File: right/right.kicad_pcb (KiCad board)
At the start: 2 copper layers, 50 parts, among them J2 USB_C_Receptacle_OUT, SW1 SW_Push, SW2 SW_SPDT, U1 STM32G0B1CBTx, U2 SRV05-4, U3 XC6206P332MR

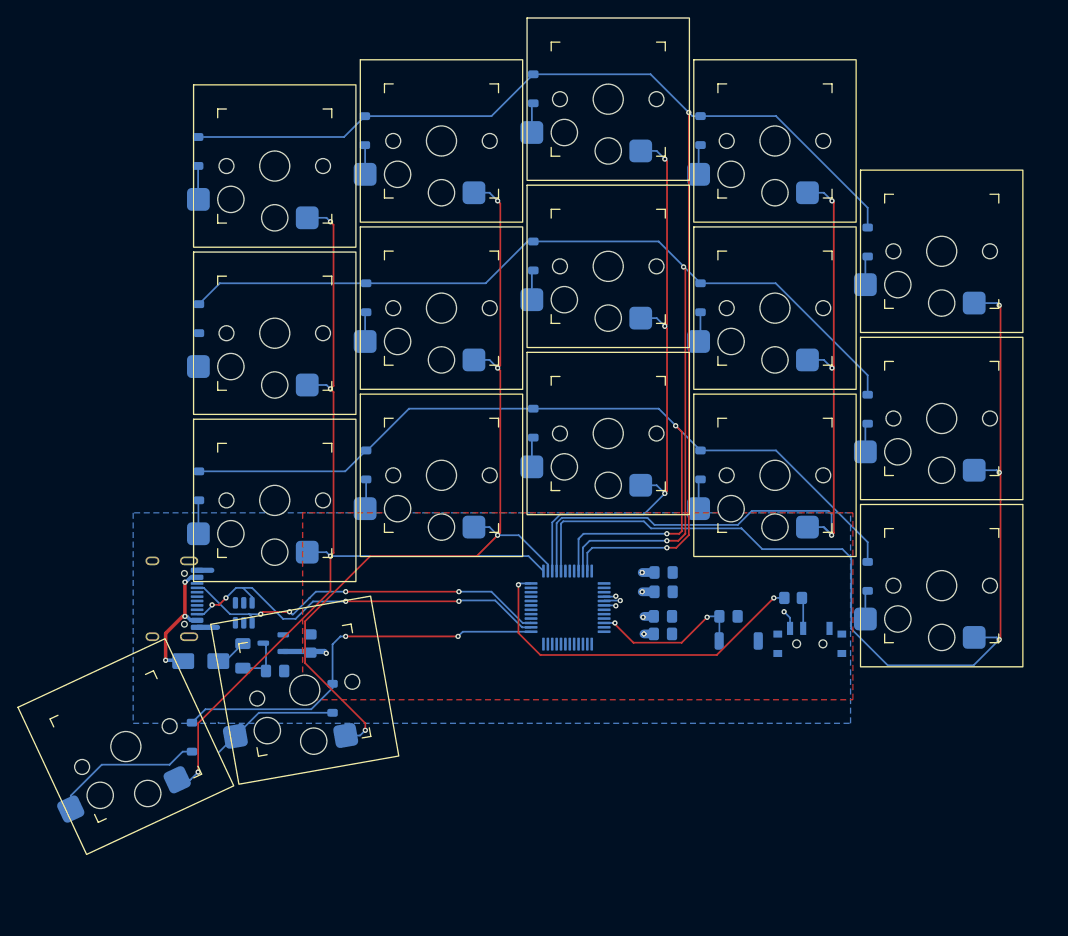
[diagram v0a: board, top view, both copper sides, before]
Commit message: unverified done right
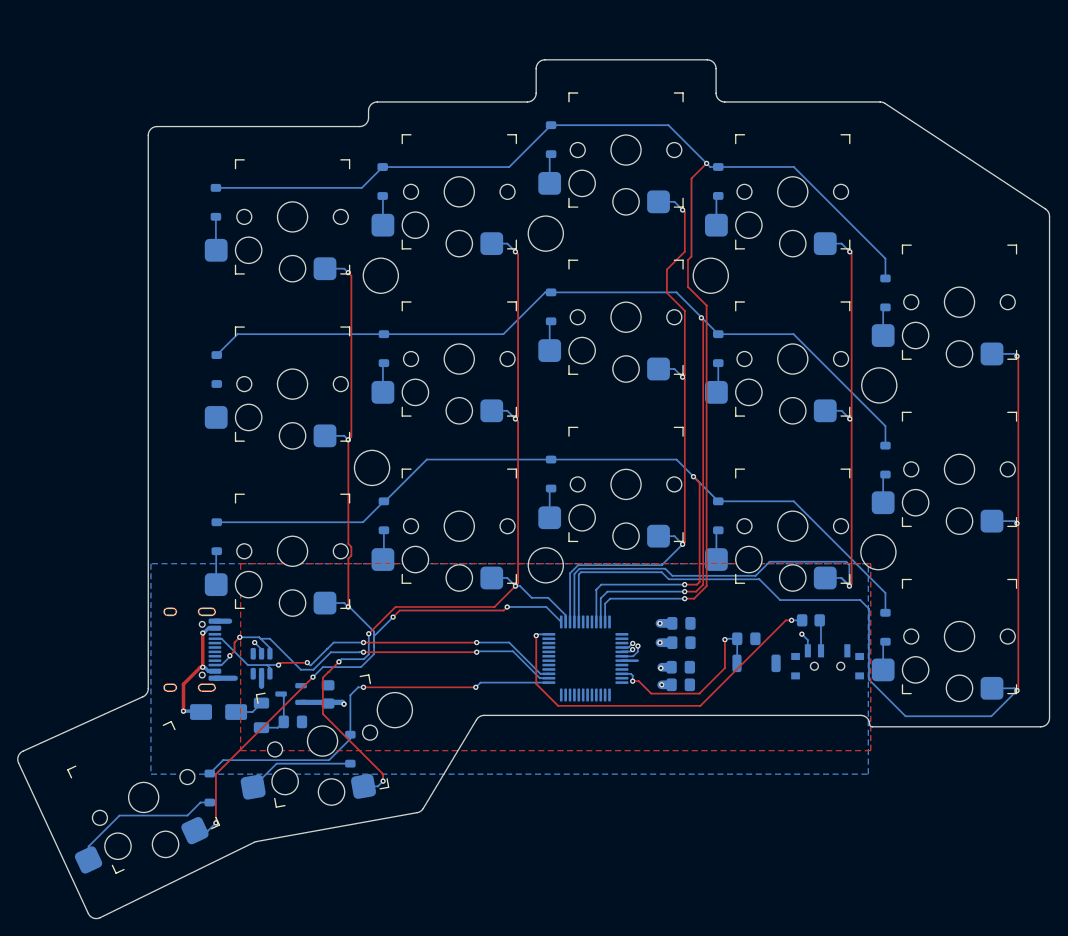
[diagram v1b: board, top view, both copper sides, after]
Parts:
- KEY1, KEY10, KEY11, KEY12, KEY13, KEY14, KEY15, KEY16, KEY17, KEY2, KEY3, KEY4, KEY5, KEY6, KEY7, KEY8, KEY9: footprint Low Profile Keyswitches:SW_Kailh_Choc_V1_HotSwap_18mm_caps -> Low Profile Keyswitches:SW_Kailh_Choc_V1_HotSwap
- moved F2 7.11 mm to (85.8, 126.1)
- moved C6 6.14 mm to (89.4, 126.8)
- moved D18 6.14 mm to (80.9, 125.7)
- moved D7 6.14 mm to (99.8, 84.3)
- moved D15 6.14 mm to (156.9, 116.1)
- moved D9 6.14 mm to (137.9, 84.3)
- moved KEY11 6.14 mm to (89.3, 107.4)
- moved KEY17 6.14 mm to (92.8, 129.0)
- moved U2 6.14 mm to (85.8, 120.2)
- moved D1 6.14 mm to (80.6, 67.6)
- moved D2 6.14 mm to (99.6, 65.3)
- moved D12 6.14 mm to (99.8, 103.4)
- moved C1 6.14 mm to (133.6, 122.6)
- moved C2 6.14 mm to (133.6, 120.6)
- moved C3 6.14 mm to (133.6, 117.8)
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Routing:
- net COL0: track 105.8 -> 110.5 mm, vias 4 -> 7
- net nRST: track 18.3 -> 21.7 mm
- net GND: track 3.99 -> 7.22 mm
- net Net-(D17-A): track 14.8 -> 12.2 mm
- net +3.3V: track 17.1 -> 19.6 mm, vias 9 -> 10
- net ROW0: track 150.5 -> 152.2 mm
- net COL2: track 67.7 -> 69.3 mm
- net BOOT0: track 41.0 -> 42.4 mm
- net COL1: track 99.5 -> 100.5 mm, vias 4 -> 6
- net TX: track 45.2 -> 45.9 mm
- net +5V: track 6.07 -> 6.58 mm
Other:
- board outline added: 117.6 x 97.9 mm

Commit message: fixed schematics
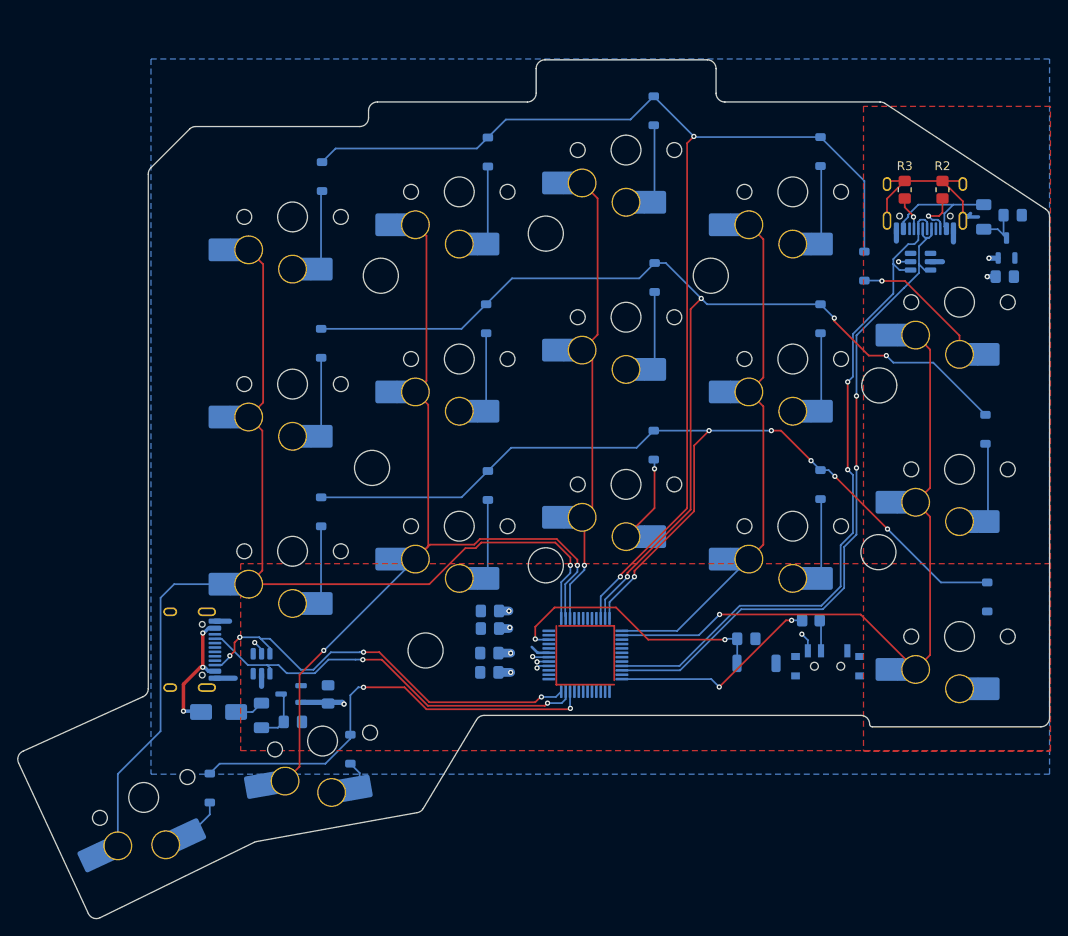
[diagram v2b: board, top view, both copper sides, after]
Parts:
- added C8: 1uF, Capacitor_SMD:C_0805_2012Metric_Pad1.18x1.45mm_HandSolder, B.Cu at (171.4, 69.1)
- added C9: 1uF, Capacitor_SMD:C_0805_2012Metric_Pad1.18x1.45mm_HandSolder, B.Cu at (170.5, 76.1)
- added F1: 1A, Fuse:Fuse_1206_3216Metric, B.Cu at (168.1, 69.3)
- added J1: USB_C_Receptacle_IN, Connector_USB:USB_C_Receptacle_HRO_TYPE-C-31-M-12, B.Cu at (161.4, 66.6)
- added R2: 5.1k, Resistor_SMD:R_0805_2012Metric_Pad1.20x1.40mm_HandSolder, F.Cu at (163.4, 66.2)
- added R3: 5.1k, Resistor_SMD:R_0805_2012Metric_Pad1.20x1.40mm_HandSolder, F.Cu at (159.1, 66.2)
- added U4: XC6206P332MR, Package_TO_SOT_SMD:SOT-23-3, B.Cu at (170.7, 72.8)
- added U5: SRV05-4, Package_TO_SOT_SMD:SOT-23-6, B.Cu at (160.9, 74.4)
- KEY1, KEY10, KEY11, KEY12, KEY13, KEY14, KEY15, KEY16, KEY17, KEY2, KEY3, KEY4, KEY5, KEY6, KEY7, KEY8, KEY9: footprint Low Profile Keyswitches:SW_Kailh_Choc_V1_HotSwap -> Keyswitches Marbastlib Choc:SW_choc_v1_HS_CPG135001S30_1u; moved to B.Cu
- moved C1 23.3 mm to (111.8, 114.2), turned to 180 degrees
- moved C4 22.6 mm to (111.8, 121.2), turned to 180 degrees
- moved C2 22.2 mm to (111.8, 116.2), turned to 180 degrees
- moved C3 21.9 mm to (111.8, 119.0), turned to 180 degrees
- moved D2 12.5 mm to (111.6, 61.9)
- moved D1 12.4 mm to (92.7, 64.7)
- moved D12 12.3 mm to (111.6, 99.9)
- moved D6 12.3 mm to (92.6, 83.7)
- moved D8 12.3 mm to (130.6, 76.2)
- moved D11 12.2 mm to (92.6, 102.9)
- moved D14 12.2 mm to (149.5, 99.8)
- moved D13 12.2 mm to (130.5, 95.3)
- moved D3 12.2 mm to (130.5, 57.2)
- moved D9 12.1 mm to (149.5, 80.9)
- moved D4 12.1 mm to (149.5, 61.9)
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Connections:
- U1 pad 13: unconnected-(U1-PA2-Pad13) -> COL0
- U1 pad 14: unconnected-(U1-PA3-Pad14) -> COL1
- U1 pad 15: unconnected-(U1-PA4-Pad15) -> COL2
- U1 pad 22: unconnected-(U1-PB10-Pad22) -> ROW0
- U1 pad 23: unconnected-(U1-PB11-Pad23) -> ROW1
- U1 pad 24: unconnected-(U1-PB12-Pad24) -> ROW2
- U1 pad 25: ROW3 -> COL3
- U1 pad 26: TX -> COL4
- U1 pad 27: RX -> unconnected-(U1-PB15-Pad27)
- U1 pad 37: COL0 -> unconnected-(U1-PA15-Pad37)
- U1 pad 38: COL1 -> unconnected-(U1-PD0-Pad38)
- U1 pad 39: COL2 -> unconnected-(U1-PD1-Pad39)
- U1 pad 40: COL3 -> unconnected-(U1-PD2-Pad40)
- U1 pad 41: COL4 -> unconnected-(U1-PD3-Pad41)
- U1 pad 45: ROW2 -> unconnected-(U1-PB6-Pad45)
- U1 pad 46: ROW1 -> ROW3
- U1 pad 47: ROW0 -> RX
- U1 pad 48: unconnected-(U1-PB9-Pad48) -> TX
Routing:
- net D-: track 0.00 -> 79.0 mm, vias 0 -> 2
- net D+: track 0.00 -> 77.4 mm, vias 0 -> 2
- net COL4: track 115.4 -> 77.9 mm, vias 3 -> 1
- net COL3: track 89.9 -> 58.7 mm, vias 3 -> 0
- net GND: track 7.22 -> 34.2 mm
- net (no net): track 0.00 -> 25.8 mm
- net BOOT0: track 42.4 -> 24.1 mm
- net COL2: track 69.3 -> 52.8 mm, vias 3 -> 1
- net ROW0: track 152.2 -> 136.3 mm
- net Net-(F1-Pad1): track 0.00 -> 14.9 mm
- net COL0: track 110.5 -> 125.2 mm, vias 7 -> 1
- net Net-(D16-A): track 17.4 -> 4.31 mm
- net Net-(D5-A): track 3.31 -> 15.6 mm, vias 0 -> 1
- net nRST: track 21.7 -> 31.3 mm
- net Net-(D17-A): track 12.2 -> 3.16 mm
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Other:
- outline, holes or cut-outs redrawn
